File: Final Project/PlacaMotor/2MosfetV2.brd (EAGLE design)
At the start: 55.9 x 39.6 mm, 23 parts, among them IC1 ATTINY44-SSU

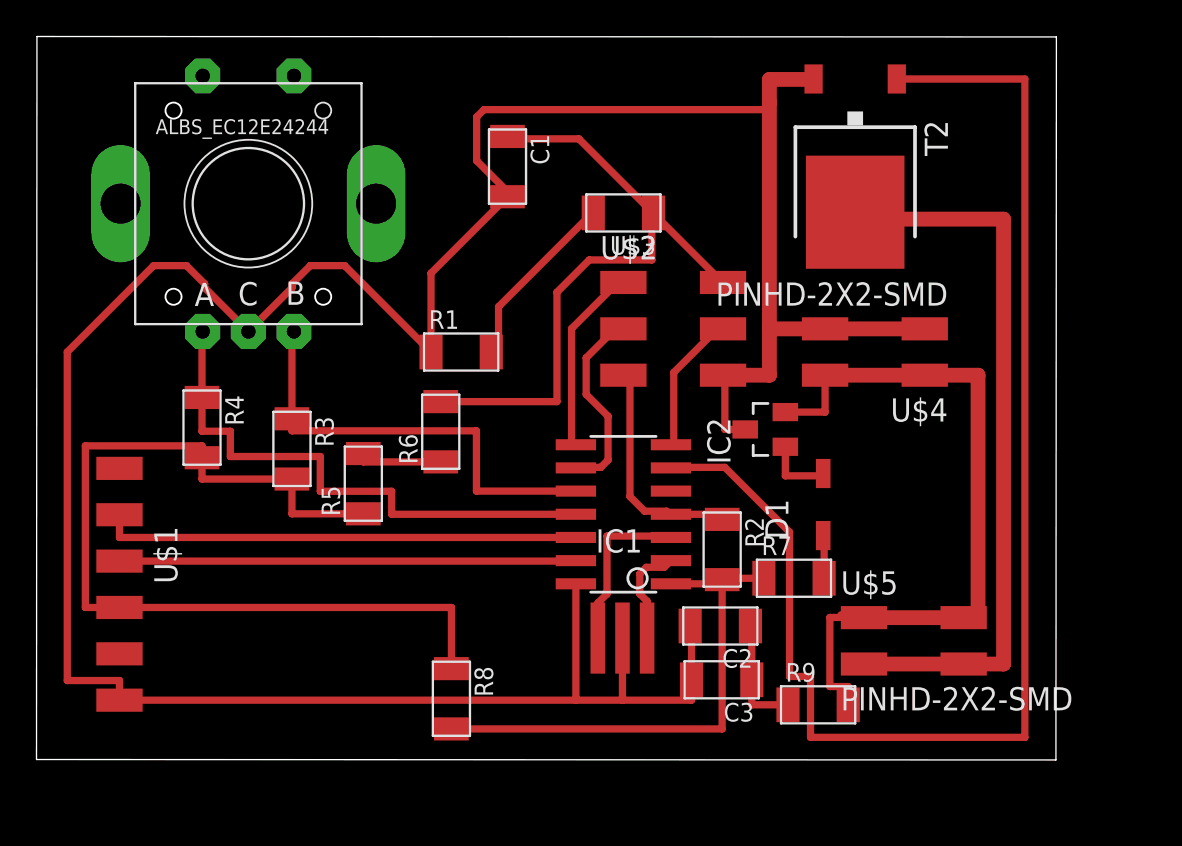
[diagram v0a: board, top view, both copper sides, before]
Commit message: lala
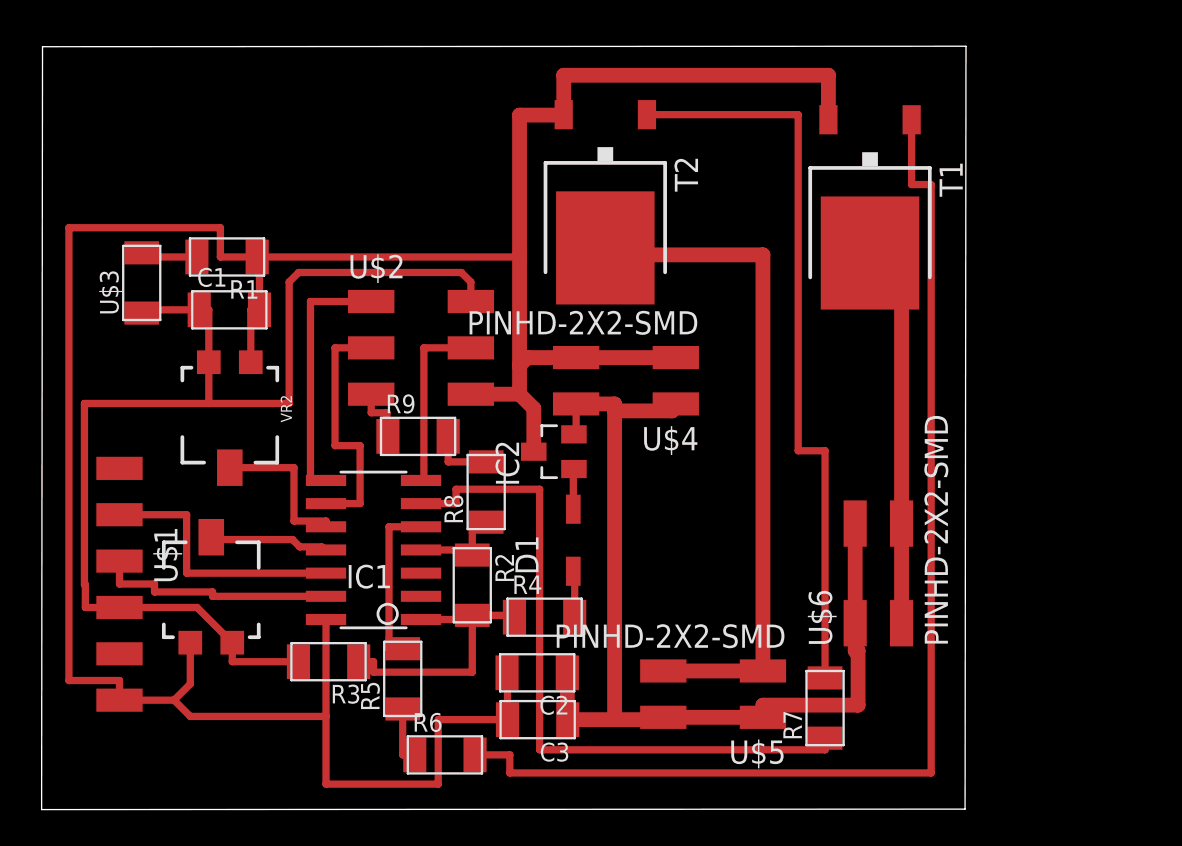
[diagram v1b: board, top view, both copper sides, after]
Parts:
- removed U$7: RESONATOR, fab:EFOBM
- added T1: (no value), fab:TO252
- added VR1, VR2: 5k, SparkFun-Resistors:TRIMPOT-SMD-5MM
- C2: value 10uF -> 0.1uF
- C3: value 0.1uF -> 10uF
- R3, R4: value 10k -> 0
- U$6: value ALBS_ENCODER_STEC12E08 -> PINHD-2X2-SMD; device Rotary Encoder:STEC12E08 -> fab:2X02SMD
- moved U$6 40.1 mm to (46.5, 9.86), turned to 90 degrees
- moved U$3 26.7 mm to (6.15, 26.0), turned to 90 degrees
- moved R9 26.4 mm to (21.3, 17.6)
- moved R4 21.5 mm to (28.2, 7.65), turned to 0 degrees
- moved R6 17.7 mm to (22.8, 0.10), turned to 0 degrees
- moved C1 17.1 mm to (10.9, 24.5), turned to 0 degrees
- moved U$2 13.9 mm to (21.3, 22.4)
- moved R1 13.8 mm to (10.8, 27.4), turned to 180 degrees
- moved D1 13.8 mm to (29.8, 11.9)
- moved R2 13.8 mm to (24.3, 9.40)
- moved T2 13.8 mm to (31.5, 30.4)
- moved IC1 13.8 mm to (18.8, 11.3)
- moved U$4 13.7 mm to (32.9, 20.6)
- moved R3 11.8 mm to (16.4, 5.21), turned to 180 degrees
- moved IC2 11.6 mm to (28.7, 16.7)
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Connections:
- removed net CRYSTAL1: IC1.3, U$7.1
- removed net CRYSTAL2: IC1.2, U$7.3
- removed net ENC1: IC1.10, R3.1, U$6.P$B
- removed net ENC2: IC1.11, R4.1, U$6.P$A
- removed net N$5: IC1.5
- new net -: IC1.2
- new net AIR: IC1.5, R5.1, R5.2, R6.1, R6.2, T1.1
- new net ANALOG: IC1.11, VR1.B
- new net ANALOG2: IC1.10, VR2.B
- new net MOSFET2: T1.3, U$6.3, U$6.4
- new net N$6: IC1.3
- net 0: now also T1.2, VR1.C, VR2.C; no longer U$6.P$C, U$7.2
- net 12V: now also U$6.1, U$6.2; no longer R9.1, R9.2
- net MOTOR: now also R7.1, R7.2
- net RST: now also R8.1, R8.2, R9.1, R9.2
- net VCC: now also R3.1, R4.1, VR1.A, VR2.A; no longer R5.1, R5.2, R6.1, R6.2, R7.1, R7.2, R8.1, R8.2
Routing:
- net AIR: track 0.00 -> 75.2 mm
- net VCC: track 123.1 -> 82.0 mm
- net ENC2: track 30.5 -> 0.00 mm
- net ENC1: track 24.4 -> 0.00 mm
- net MOSFET2: track 0.00 -> 22.0 mm
- net TX: track 25.1 -> 13.2 mm
- net RX: track 26.3 -> 14.5 mm
- net CRYSTAL1: track 9.33 -> 0.00 mm
- net ANALOG2: track 0.00 -> 8.51 mm
- net 12V: track 47.7 -> 54.6 mm
- net N$1: track 10.1 -> 3.25 mm
- net 0: track 160.3 -> 153.4 mm
- net ANALOG: track 0.00 -> 6.59 mm
- net CRYSTAL2: track 5.69 -> 0.00 mm
- net MOTOR: track 75.2 -> 78.6 mm
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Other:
- board size 55.9 x 39.6 mm -> 50.6 x 41.8 mm
